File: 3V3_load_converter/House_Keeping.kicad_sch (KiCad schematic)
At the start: 4 parts, among them Q7 SI2302DDS-T1-GE3, U15 CD4051BPWR, U16 CD4051BPWR

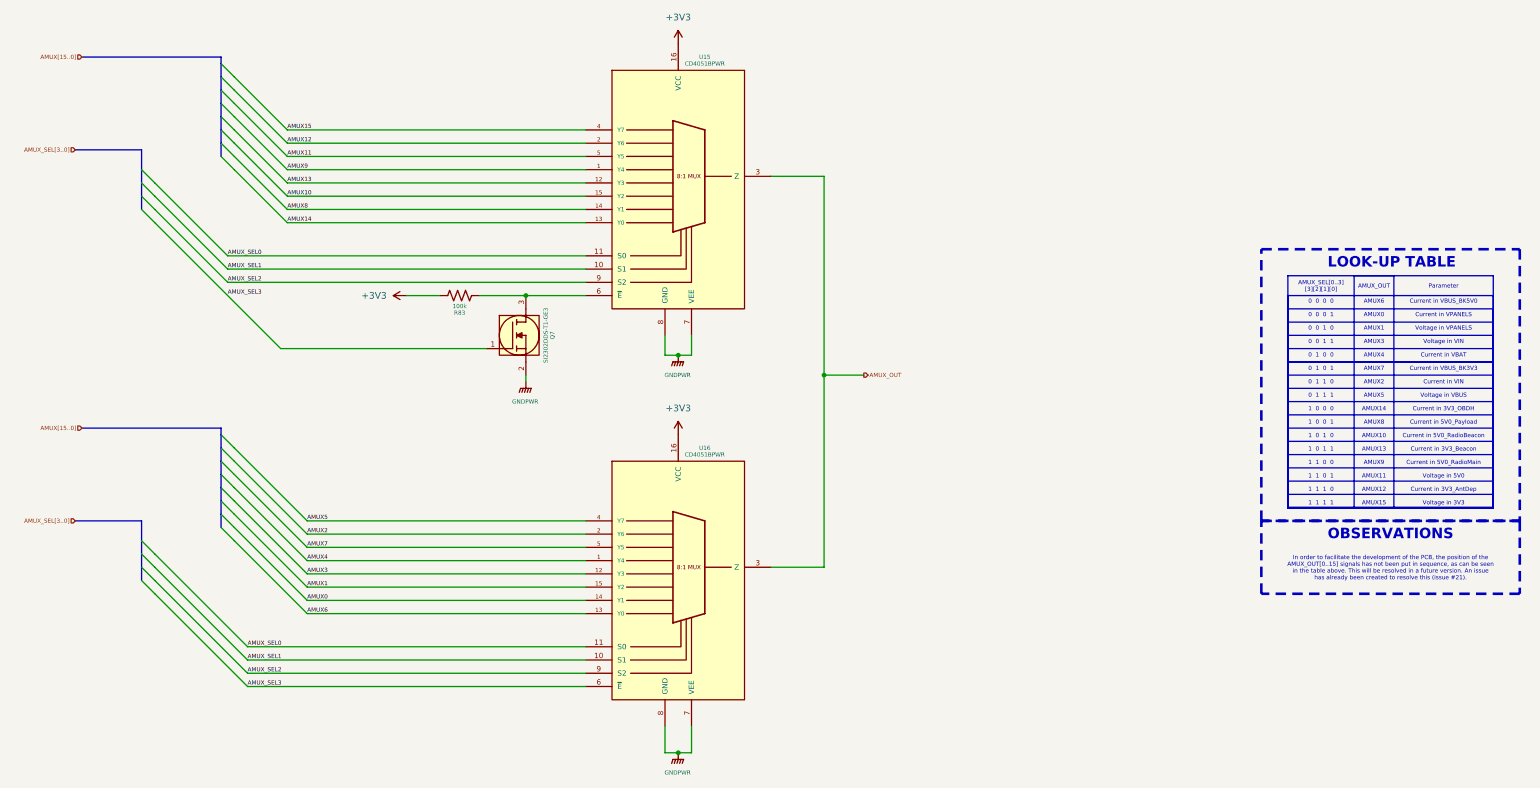
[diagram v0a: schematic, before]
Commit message: update
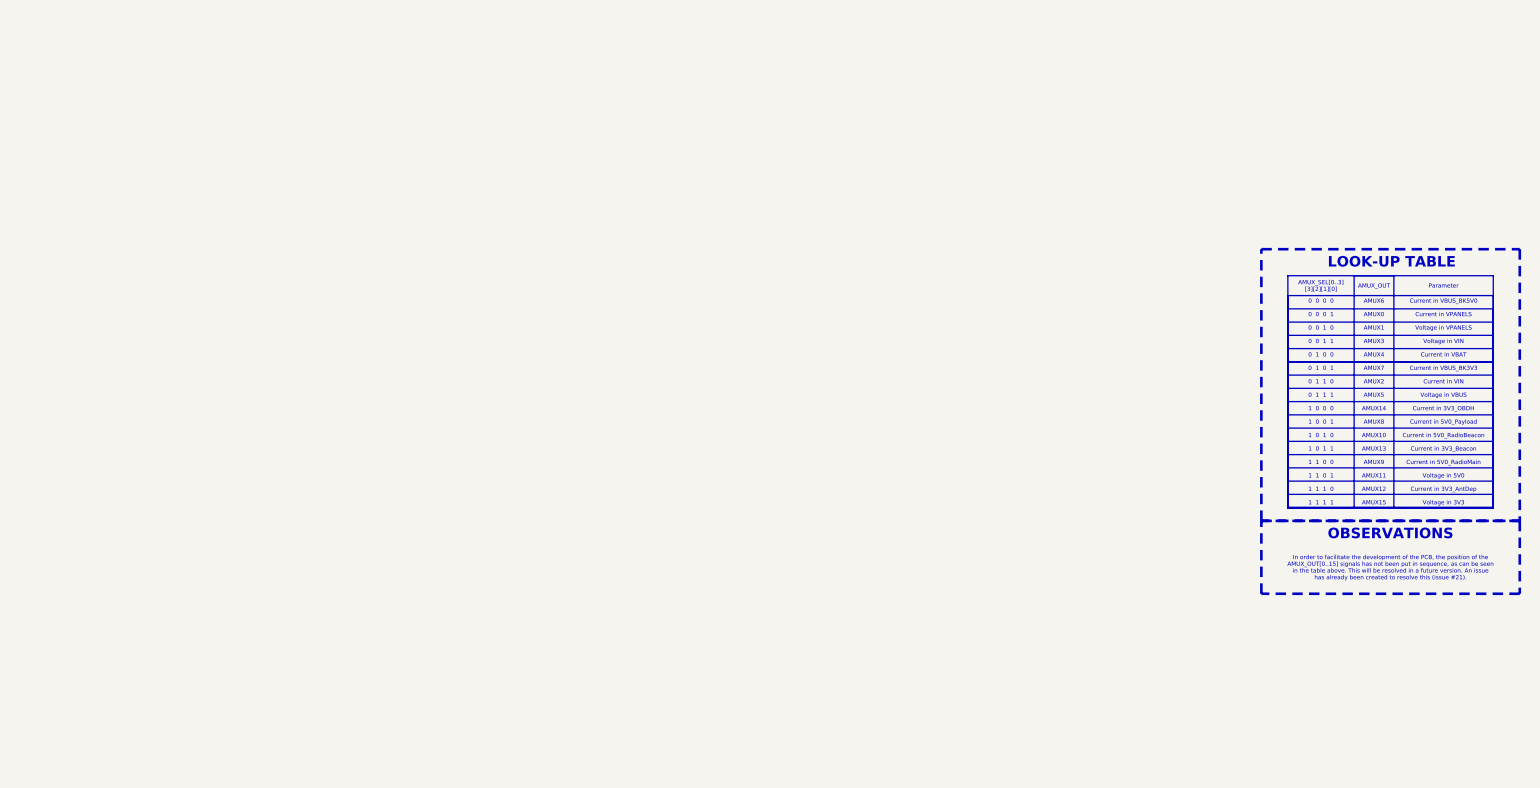
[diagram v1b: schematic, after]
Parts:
- removed Q7: SI2302DDS-T1-GE3, footprints:SI2302DDS-T1-GE3, symbol SI2302DDS-T1-GE3:SI2302DDS-T1-GE3
- removed R83: 100k, footprints:RES0603, symbol CRCW0603100KFKEAHP:CRCW0603100KFKEAHP
- removed U15, U16: CD4051BPWR, footprints:CD4051BPWR, symbol CD4051BPWR:CD4051BPWR
